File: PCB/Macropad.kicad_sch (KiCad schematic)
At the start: 9 parts, among them SW1 SW_Push, SW2 SW_Push, SW3 SW_Push, SW4 SW_Push, SW5 SW_Push, SW6 SW_Push, U1 XIAO-RP2040-DIP

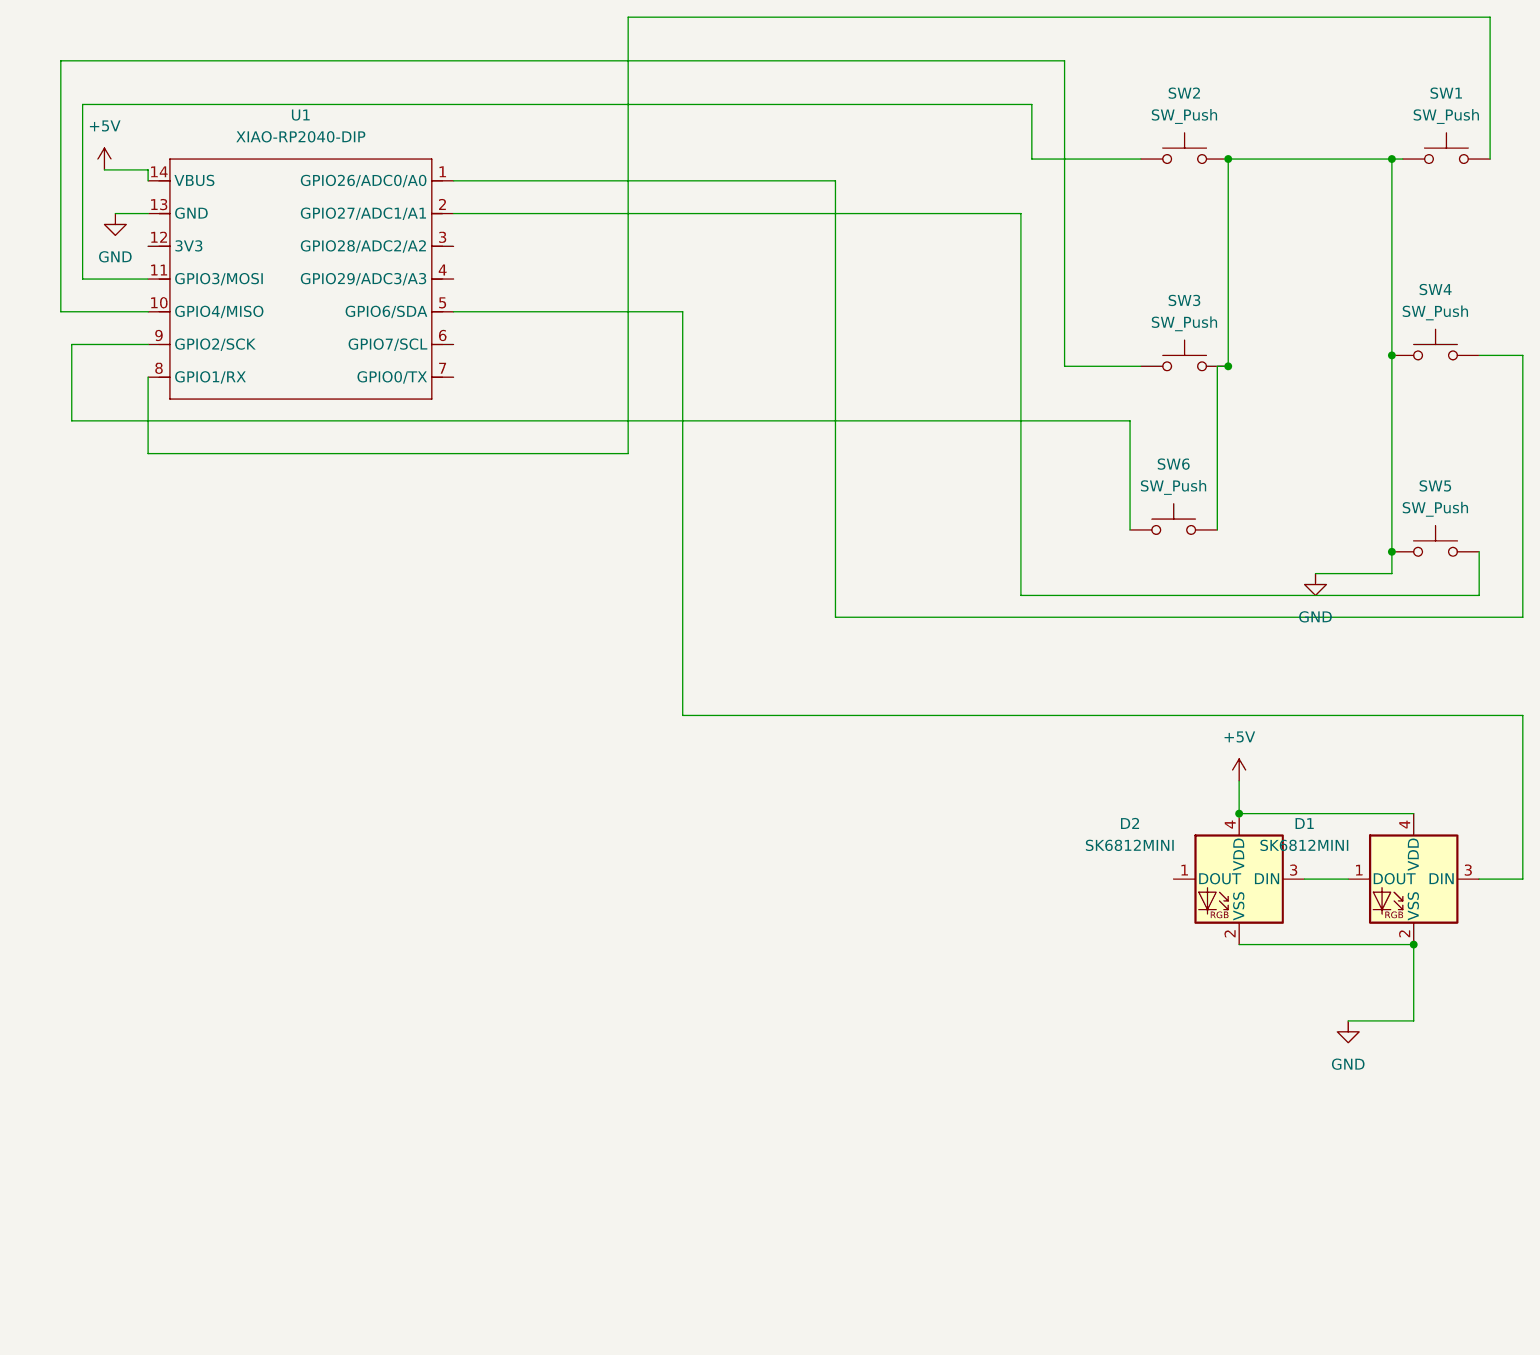
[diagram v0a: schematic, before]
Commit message: OLED
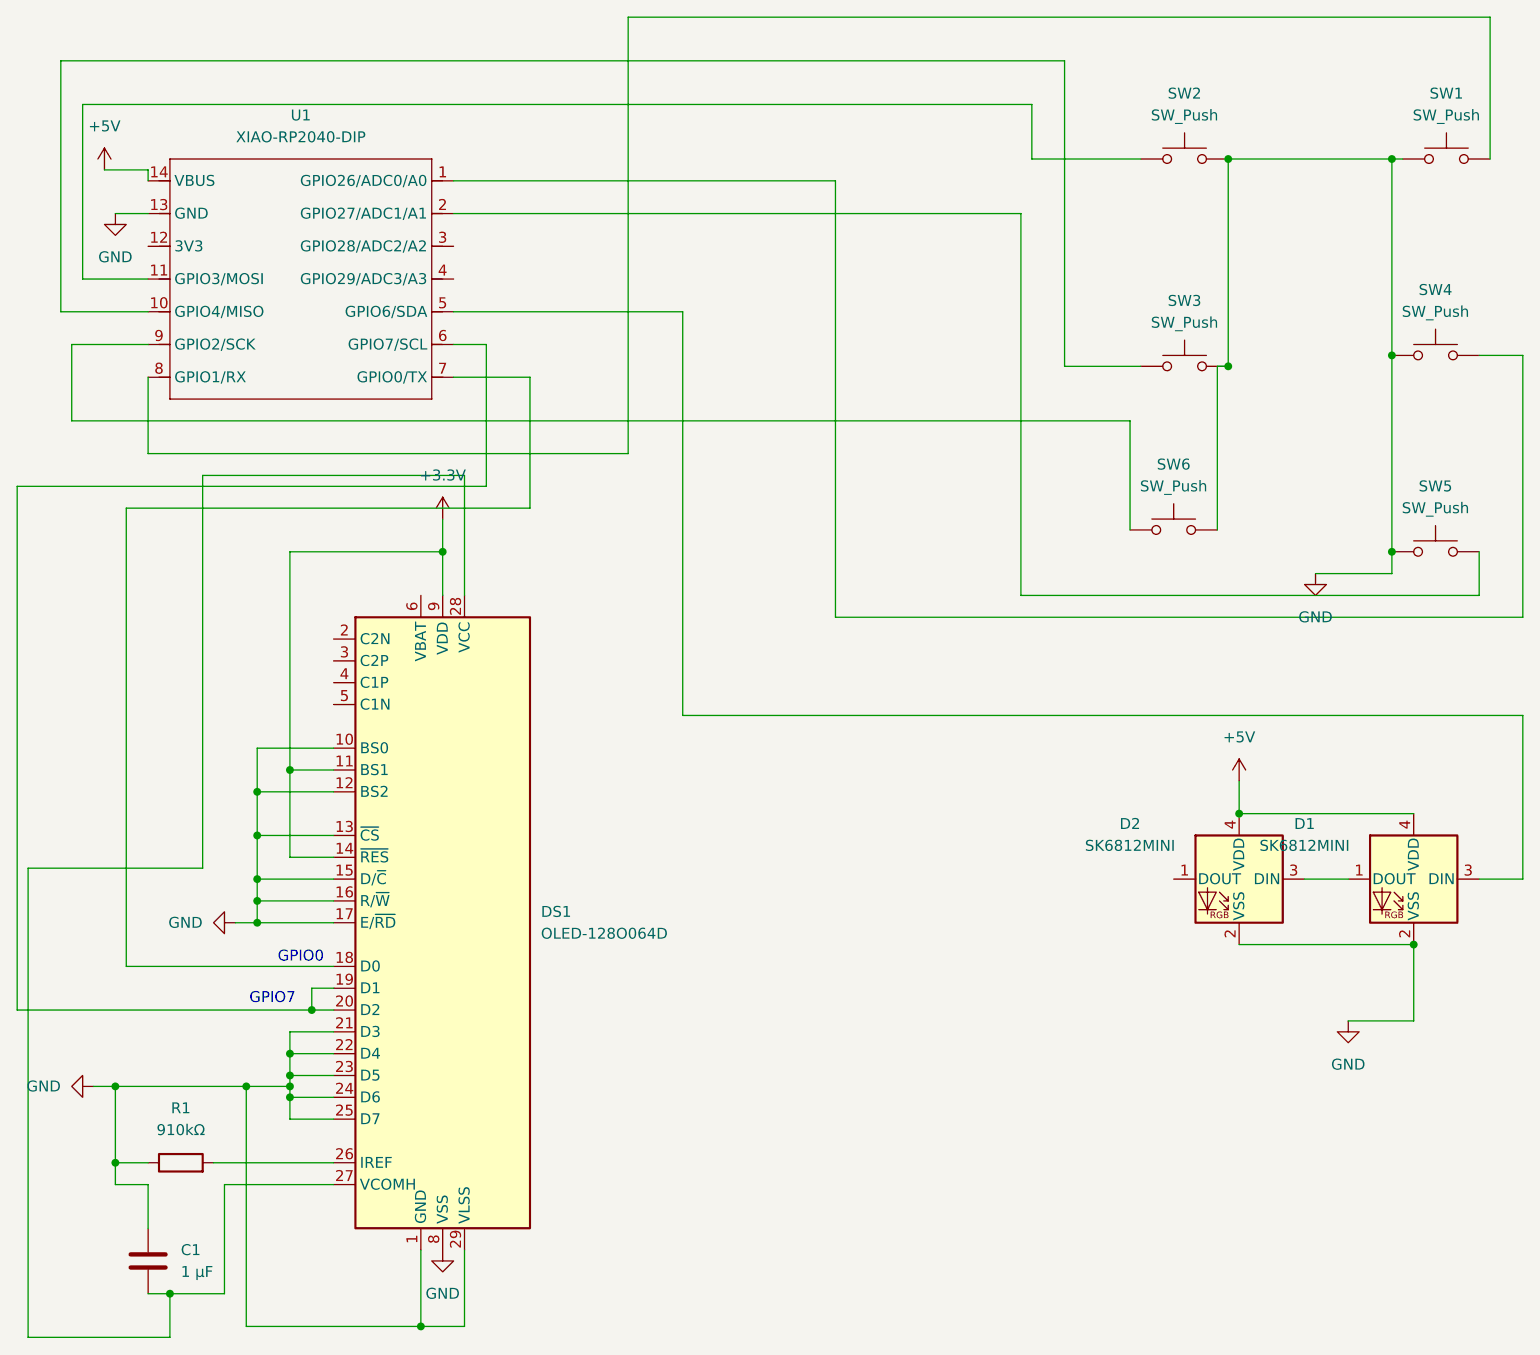
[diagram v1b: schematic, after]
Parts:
- added C1: 1 µF, Capacitor_SMD:C_0402_1005Metric, symbol Device:C
- added DS1: OLED-128O064D, Display:OLED-128O064D, symbol Display_Graphic:OLED-128O064D
- added R1: 910kΩ, Resistor_THT:R_Axial_DIN0204_L3.6mm_D1.6mm_P1.90mm_Vertical, symbol Device:R
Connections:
- net GND: now also C1.1, DS1.1 (GND), DS1.10 (BS0), DS1.12 (BS2), DS1.13 (~{CS}), DS1.15 (D/~{C}), DS1.16 (R/~{W}), DS1.17 (E/~{RD}), DS1.21 (D3), DS1.22 (D4), DS1.23 (D5), DS1.24 (D6), DS1.25 (D7), DS1.29 (VLSS), DS1.30 (GND), DS1.8 (VSS), R1.1
- net at U1.6 (GPIO7/SCL): now also DS1.19 (D1), DS1.20 (D2)
- net at U1.7 (GPIO0/TX): now also DS1.18 (D0)
- new net: C1.2, DS1.27 (VCOMH), DS1.28 (VCC)
- new net: DS1.26 (IREF), R1.2
- new net +3.3V: DS1.11 (BS1), DS1.14 (~{RES}), DS1.9 (VDD)
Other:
- note added: "GPIO0"
- note added: "GPIO7"
